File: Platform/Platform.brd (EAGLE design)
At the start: 97.8 x 36.8 mm, 30 parts, among them U1 LCD-16X2NOSILK, U2 LM2574N, X1 USBSMD, Y1 RESONATORSMD

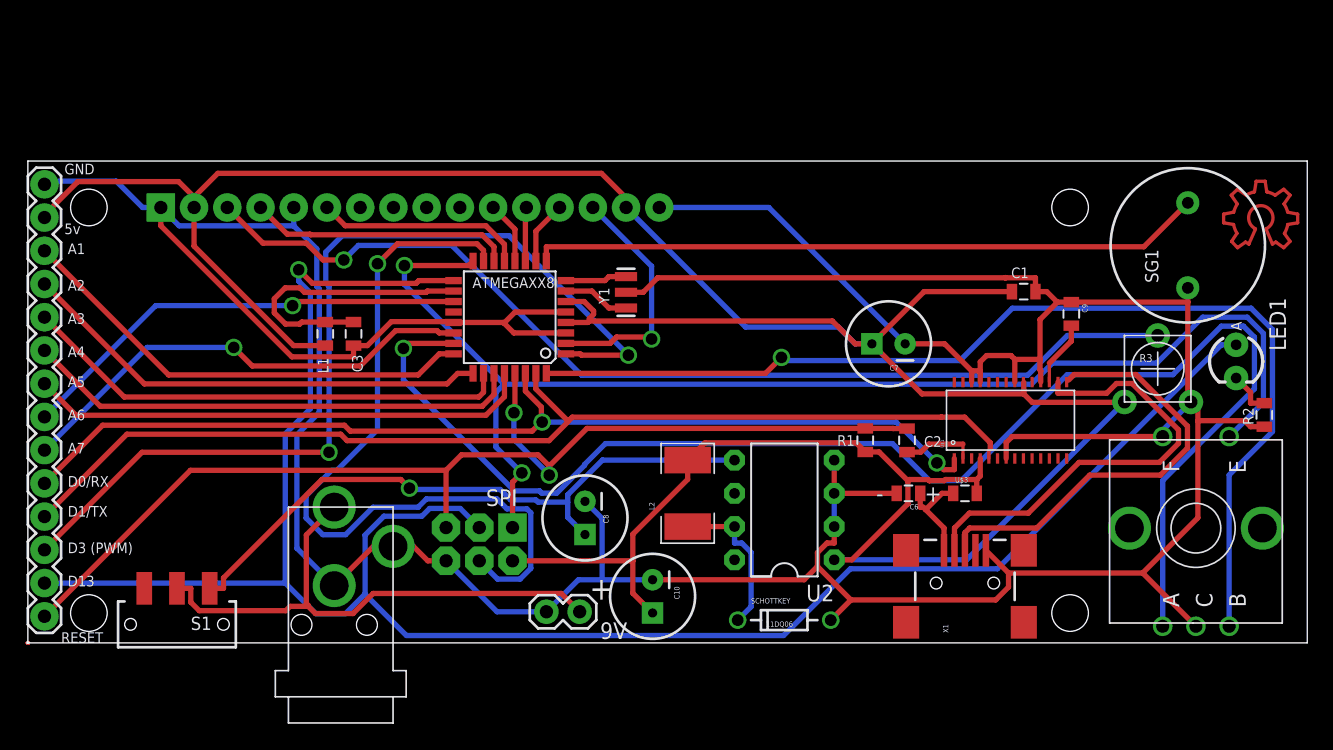
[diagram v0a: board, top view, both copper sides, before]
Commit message: prototype 3
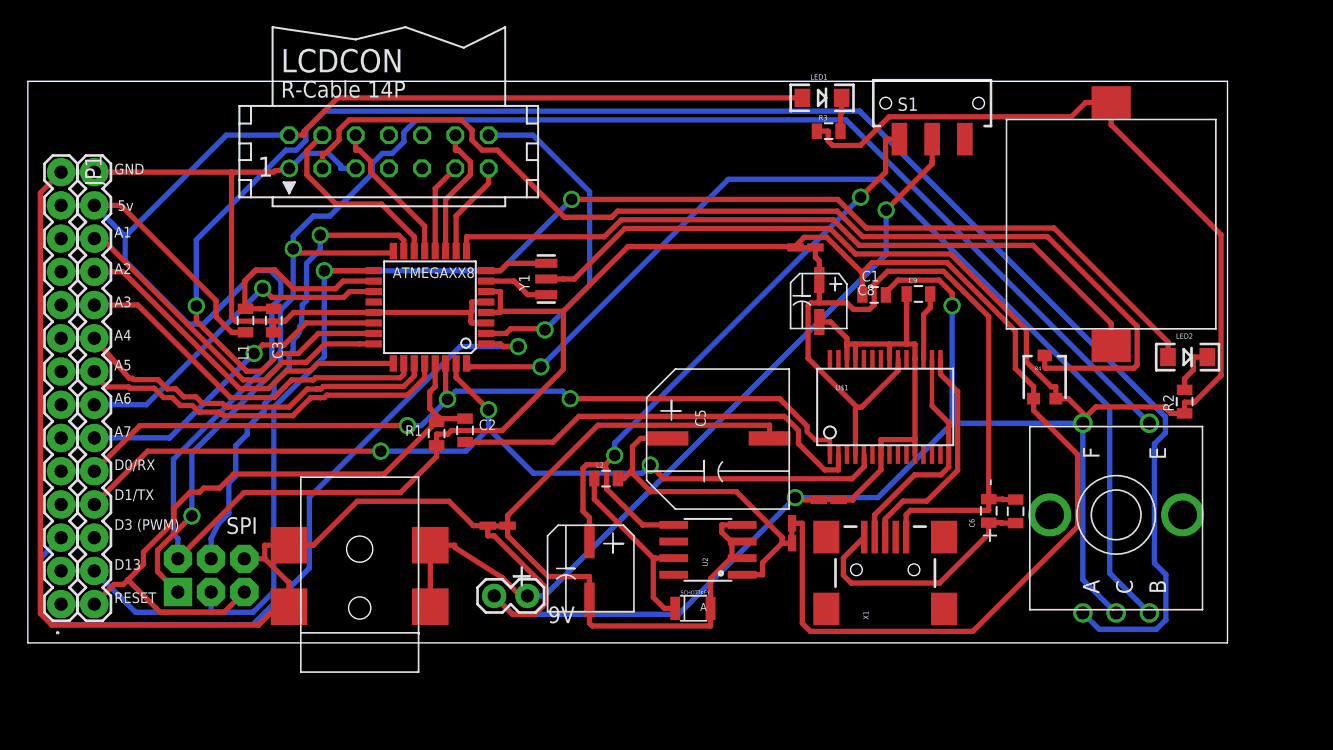
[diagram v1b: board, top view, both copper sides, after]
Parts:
- removed C10: 220uf, SparkFun:CPOL-RADIAL-100UF-25V
- removed C7: 4.7uf, SparkFun:CPOL-RADIAL-100UF-25V
- removed LOGO1: OSHW_LOGO_10MIL, ohw-logo:OSHW_10X200_NOTEXT_COPPER
- removed SG1: BUZZERPTH, SparkFun:BUZZER-12MM
- removed U1: LCD-16X2NOSILK, SparkFun:LCD-16X2_NOSILK
- added C4: 68uf, Dustin:F80
- added C5: 120uf, Dustin:10X8CAP
- added JP1: M14B, Dustin:1X14B
- added LCDCON: (no value), con-harting:CON14
- added LED2: RED, SparkFun:LED-1206
- added LINK1, LINK2, LINK3, LINK4: LINK, Dustin:ISOLATOR
- added R4: TRIMPOTSMD, SparkFun:TRIMPOT-3MM
- added SG2: BUZZERSMD, SparkFun:BUZZER-CMT1603
- C8: value 22uf -> 4.7uf; device SparkFun:CPOL-RADIAL-100UF-25V -> Dustin:CAP-B
- L2: value 330uH -> 100uH; device SparkFun:INDUCTOR-1206 -> SparkFun:0805
- LED1: value (none) -> GRN; device SparkFun:LED3MM -> SparkFun:LED-1206
- R3: value 10k -> 220; device SparkFun:TRIM_POT_PTH -> SparkFun:0805
- SCHOTTKEY: value 11DQ06 -> (none); device SparkFun:DIODE-ZENER -> Dustin:SOD-123
- U$1: value FT232RL -> FT232RLSSOP; device Dustin:TSSOP28 -> Dustin:SSOP28
- U$4: value DCJACK -> DCJACKSMD; device Dustin:DCPOWERSOCKETPJ-019 -> Dustin:JACK-SMD
- U2: device Dustin:8DILL -> Dustin:SOIC8
- moved S1 70.1 mm to (69.1, 41.3), turned to 0 degrees
- moved LED1 37.5 mm to (60.7, 41.7), turned to 0 degrees
- moved C2 33.8 mm to (33.4, 16.2)
- moved R1 32.8 mm to (31.2, 16.0)
- moved R3 31.0 mm to (61.2, 39.1)
- moved C8 24.4 mm to (60.5, 26.2), turned to 0 degrees
- moved SPI 20.6 mm to (14.0, 5.16), turned to 0 degrees
- moved U$4 12.9 mm to (25.4, -2.33), turned to 0 degrees
- moved C9 11.8 mm to (68.1, 26.7), turned to 0 degrees
- moved C1 11.4 mm to (64.7, 26.6)
- moved U$1 9.96 mm to (65.5, 18.0), turned to 0 degrees
- moved SCHOTTKEY 7.06 mm to (50.8, 2.54)
- moved U2 6.59 mm to (52.0, 7.11)
- moved L2 6.34 mm to (44.2, 12.6), turned to 0 degrees
- moved C6 6.28 mm to (73.4, 10.1), turned to 90 degrees
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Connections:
- removed net CTS: U$1.11
- new net FTDI-GND: C8.-, C9.1, LINK4.P$2, U$1.11, U$1.18, U$1.21, U$1.25, U$1.26, U$1.7
- new net FTDI-VCC: C6.-, C8.+, LINK3.P$1, U$1.20, U$1.4, U$3.2, X1.GND
- new net GNDLINK: C4.-, C5.-, LINK2.P$1, SCHOTTKEY.ANODE, U2.2, U2.3, U2.4
- new net N$7: LED1.C, R3.2
- new net VCCLINK: C5.+, L2.2, LINK1.P$1, U2.1
- net A1: now also JP1.3
- net A2: now also JP1.4
- net A3: now also JP1.5
- net A4: now also JP1.6
- net A5: now also JP1.7
- net A6: now also JP1.8
- net A7: now also JP1.9
- net CONTRAST: now also LCDCON.3, R4.2; no longer R3.2, U1.3
- net D10: now also LCDCON.4; no longer U1.4
- net D13/SCK: now also JP1.13, LED2.A; no longer LED1.A
- net D3: now also JP1.12
- net D4: now also LCDCON.14; no longer U1.14
- net D5: now also SG2.P$2; no longer SG1.-
- net D6: now also LCDCON.13; no longer U1.13
- net D7: now also LCDCON.12; no longer U1.12
- net D8: now also LCDCON.11; no longer U1.11
- net D9: now also LCDCON.6; no longer U1.6
- net GND: now also JP1.1, LCDCON.1, LCDCON.5, LINK2.P$2, LINK4.P$1, R3.1, R4.3, SG2.P$1; no longer C10.2, C6.-, C7.2, C8.2, C9.1, R3.3, SCHOTTKEY.P$2, SG1.+, U$1.18, U$1.21, U$1.25, U$1.26, U$1.7, U1.1, U1.16, U1.5, U2.2, U2.3, U2.4, X1.GND
- net N$2: now also LED2.C; no longer LED1.K
- net N$3: now also L2.1, SCHOTTKEY.CATHODE; no longer L2.P$1, SCHOTTKEY.P$1
- net RAW: now also C4.+; no longer C8.1
- net RAW_IN: now also U$4.1A, U$4.1B; no longer U$4.1C
- net RESET: now also JP1.14
- net RX: now also JP1.10
- net TX: now also JP1.11
- net VCC: now also JP1.2, LCDCON.2, LED1.A, LINK1.P$2, LINK3.P$2, R4.1; no longer C10.1, C7.1, L2.P$2, R3.1, U$1.20, U$1.4, U$3.2, U1.15, U1.2, U2.1
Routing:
- net FTDI-VCC: track 0.00 -> 65.2 mm
- net GNDLINK: track 0.00 -> 57.8 mm
- net RESET: track 86.6 -> 53.2 mm, vias 2 -> 0
- net D13/SCK: track 155.3 -> 122.1 mm, vias 1 -> 2
- net FTDI-GND: track 0.00 -> 33.2 mm
- net DTR: track 5.71 -> 32.8 mm
- net A0: track 108.1 -> 134.2 mm
- net VCC: track 236.7 -> 262.9 mm
- net VCCLINK: track 0.00 -> 25.6 mm
- net D11/MOSI: track 60.1 -> 35.5 mm
- net D12/MISO: track 99.6 -> 119.6 mm
- net RAW_IN: track 42.3 -> 62.0 mm, vias 0 -> 1
- net GND: track 331.7 -> 350.1 mm, vias 0 -> 2
- net N$4: track 34.4 -> 17.7 mm
- net N$5: track 33.8 -> 17.5 mm
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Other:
- board size 97.8 x 36.8 mm -> 91.7 x 42.9 mm
